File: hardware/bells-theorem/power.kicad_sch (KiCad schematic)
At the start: 12 parts, among them J1 Conn_02x05_Odd_Even, U2 R-78B5.0-2.0, U3 ADP150-3.3

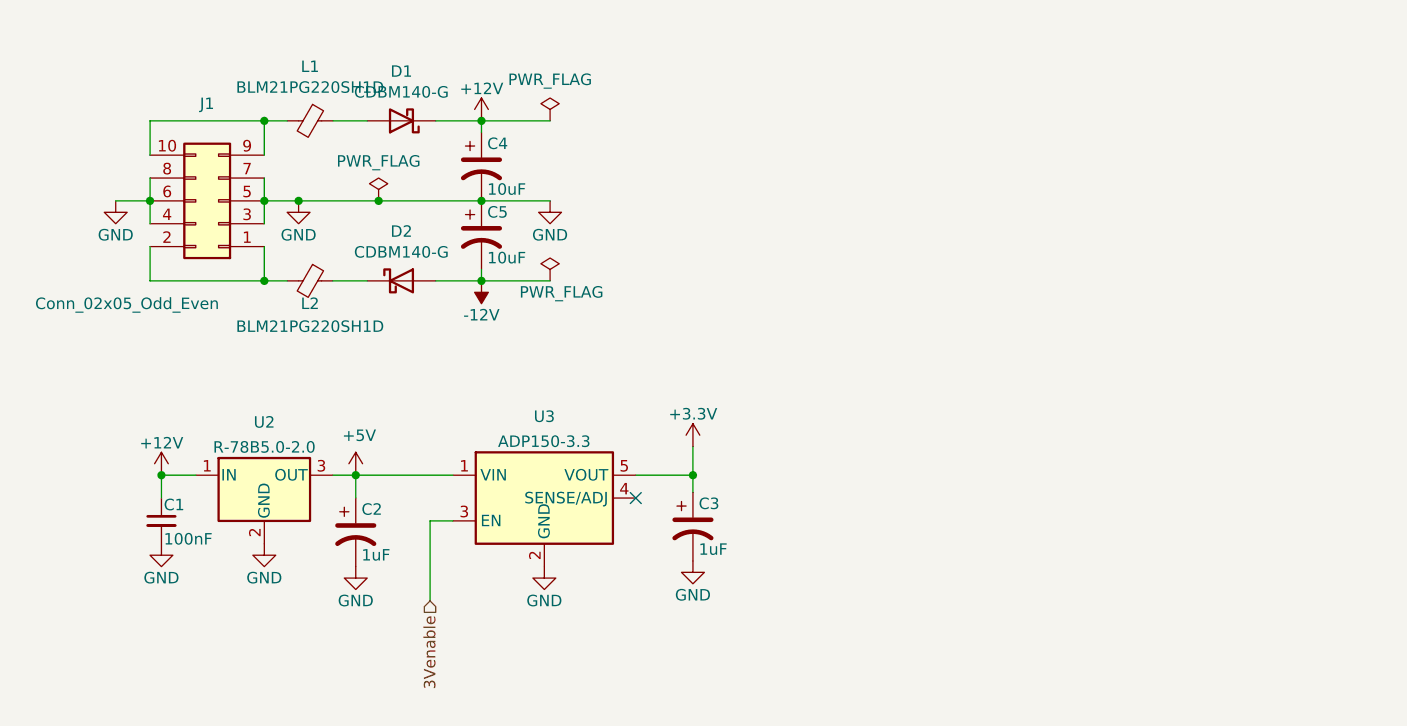
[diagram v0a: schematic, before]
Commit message: last hardware / software updates
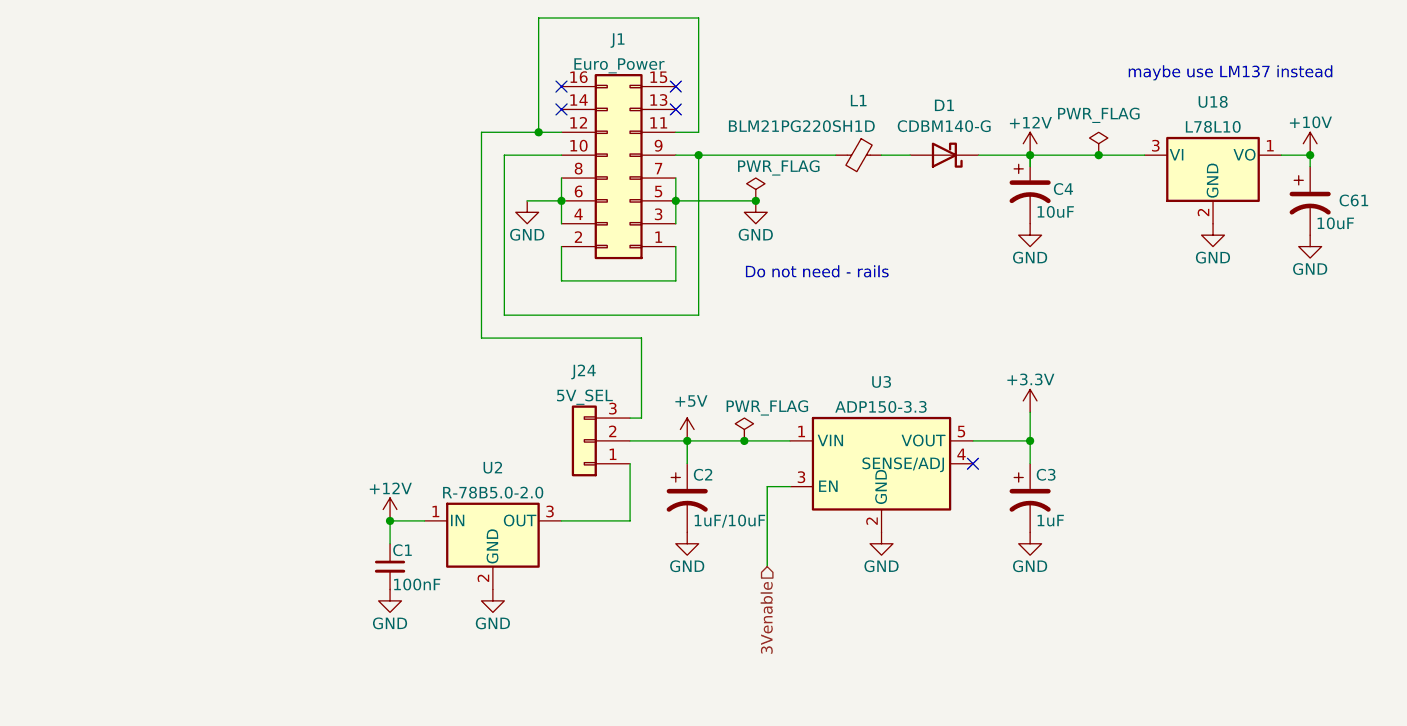
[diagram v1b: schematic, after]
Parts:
- removed C5: 10uF, Capacitor_THT:CP_Radial_D5.0mm_P2.50mm, symbol Device:C_Polarized_US
- removed D2: CDBM140-G, Diode_SMD:D_SMA-SMB_Universal_Handsoldering, symbol Device:D_Schottky
- removed J1: Conn_02x05_Odd_Even, Connector_IDC:IDC-Header_2x05_P2.54mm_Vertical, symbol Connector_Generic:Conn_02x05_Odd_Even
- removed L2: BLM21PG220SH1D, Inductor_SMD:L_0805_2012Metric_Pad1.15x1.40mm_HandSolder, symbol Device:FerriteBead_Small
- added C61: 10uF, Capacitor_THT:CP_Radial_D5.0mm_P2.50mm, symbol Device:C_Polarized_US
- added J1: Euro_Power, Connector_IDC:IDC-Header_2x08_P2.54mm_Vertical, symbol Connector_Generic:Conn_02x08_Odd_Even
- added J24: 5V_SEL, Connector_PinHeader_2.54mm:PinHeader_1x03_P2.54mm_Vertical, symbol Connector_Generic:Conn_01x03
- added U18: L78L10, Package_TO_SOT_THT:TO-92_Inline_Wide, symbol Regulator_Linear:L78L10_TO92
- C2: value 1uF -> 1uF/10uF
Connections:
- net +12V: now also U18.3 (VI)
- net +5V: now also J24.2 (Pin_2); no longer U2.3 (OUT)
- net GND: now also C61.2, J1.3 (Pin_3), J1.4 (Pin_4), J1.5 (Pin_5), J1.6 (Pin_6), J1.7 (Pin_7), J1.8 (Pin_8), U18.2 (GND)
- net at L1.2: now also J1.10 (Pin_10), J1.9 (Pin_9)
- new net: J1.1 (Pin_1), J1.2 (Pin_2)
- new net: J1.11 (Pin_11), J1.12 (Pin_12), J24.3 (Pin_3)
- new net: J24.1 (Pin_1), U2.3 (OUT)
- new net +10V: C61.1, U18.1 (VO)
- no-connect marks 1 -> 5
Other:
- note added: "Do not need - rails"
- note added: "maybe use LM137 instead"
- moved on the sheet: C1, C2, C3, C4, D1, L1, U2, U3
